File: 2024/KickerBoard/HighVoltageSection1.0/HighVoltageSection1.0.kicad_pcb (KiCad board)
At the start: 2 copper layers, 59.8 x 28.9 mm, 17 parts, among them J10 Conn_01x02_Socket, J3 Conn_01x02_Socket, J4 Conn_01x02_Socket, J6 Conn_01x02_Socket, J7 Conn_01x02_Socket, J8 Conn_01x04_Socket, J9 Conn_01x04_Socket, Q2 NMOS, Q3 NMOS

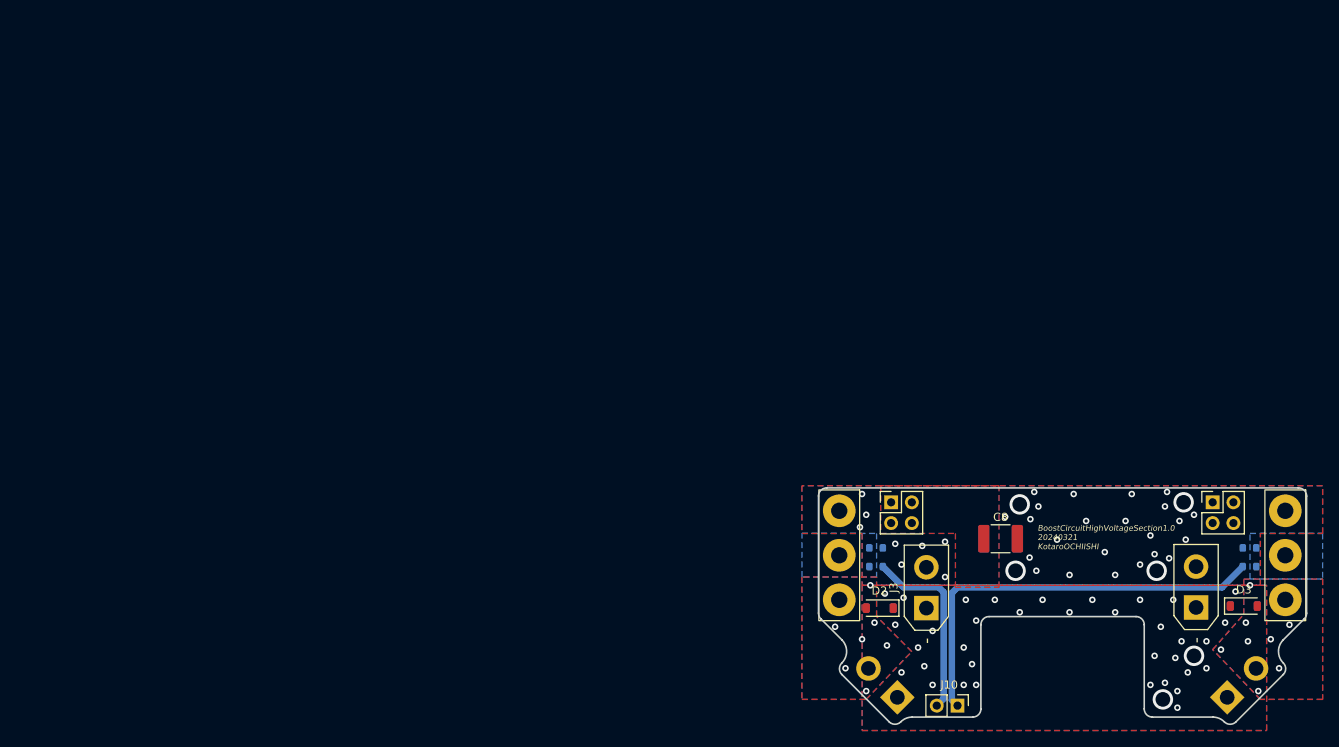
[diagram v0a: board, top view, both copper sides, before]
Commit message: add Kick&Sub
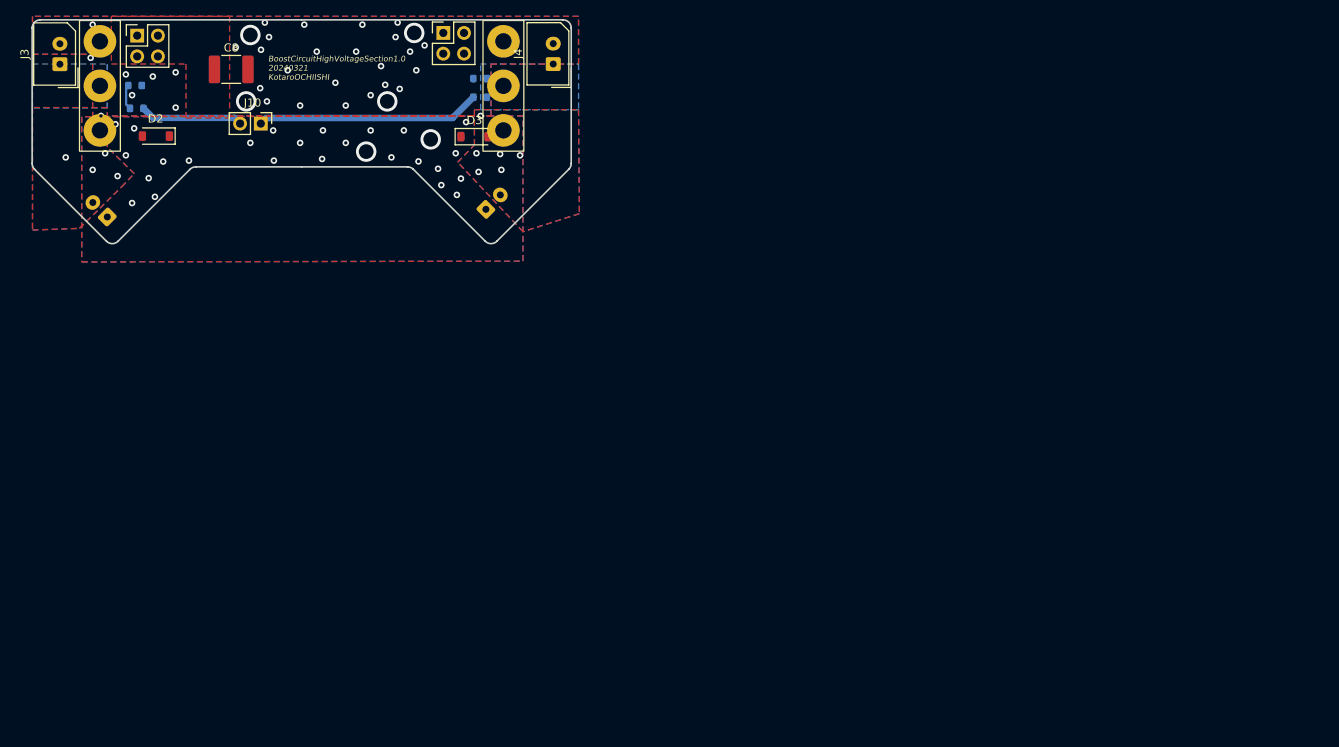
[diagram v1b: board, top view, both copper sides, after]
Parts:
- J3, J4, J6, J7: footprint Connector_AMASS:AMASS_XT30UPB-F_1x02_P5.0mm_Vertical -> Connector_Molex:Molex_SPOX_5267-02A_1x02_P2.50mm_Vertical
- moved J3 125.3 mm to (-29.6, -8.27)
- moved J6 113.2 mm to (-23.8, 10.4)
- moved Q3 111.7 mm to (24.7, -5.62)
- moved J10 111.1 mm to (-5.00, -1.00)
- moved C8 110.3 mm to (-8.63, -7.63)
- moved D3 110.3 mm to (21.1, 0.60)
- moved G*** 110.3 mm to (2.00, -5.87)
- moved J9 110.3 mm to (17.3, -12.1)
- moved R10 110.3 mm to (21.8, -4.22)
- moved R11 110.3 mm to (21.8, -6.51)
- moved J7 108.7 mm to (22.6, 9.50)
- moved J8 108.6 mm to (-20.1, -11.8)
- moved Q2 107.2 mm to (-24.7, -5.62)
- moved R9 106.9 mm to (-20.4, -5.67)
- moved R8 106.5 mm to (-20.2, -2.87)
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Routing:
- net CHIP: track 51.0 -> 27.4 mm
- net STRAIGHT: track 23.0 -> 12.6 mm
- net GATE1: track 0.00 -> 3.10 mm
- net VOUT: vias 37 -> 27
- net OUTGND2: vias 8 -> 6
- net OUTGND1: vias 7 -> 5
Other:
- board size 59.8 x 28.9 mm -> 66 x 27.4 mm

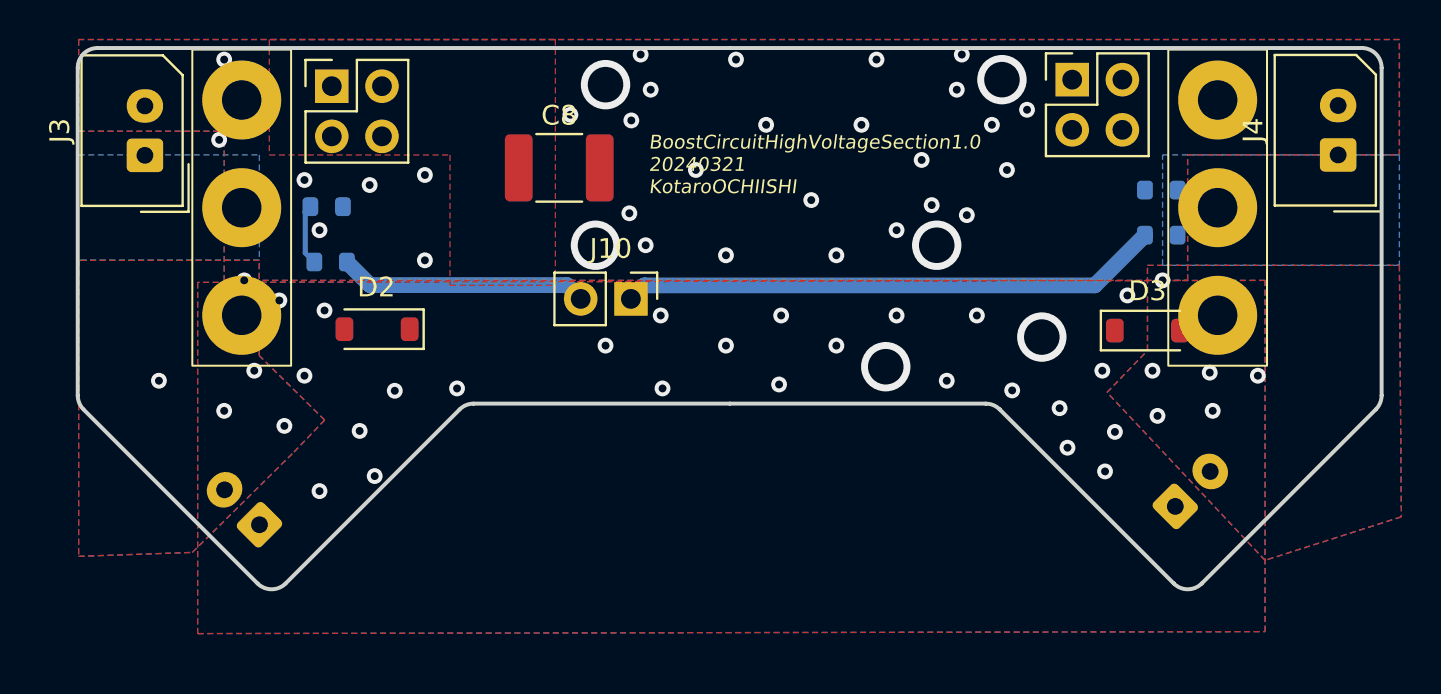
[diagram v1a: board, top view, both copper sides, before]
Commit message: add Kick&Sub
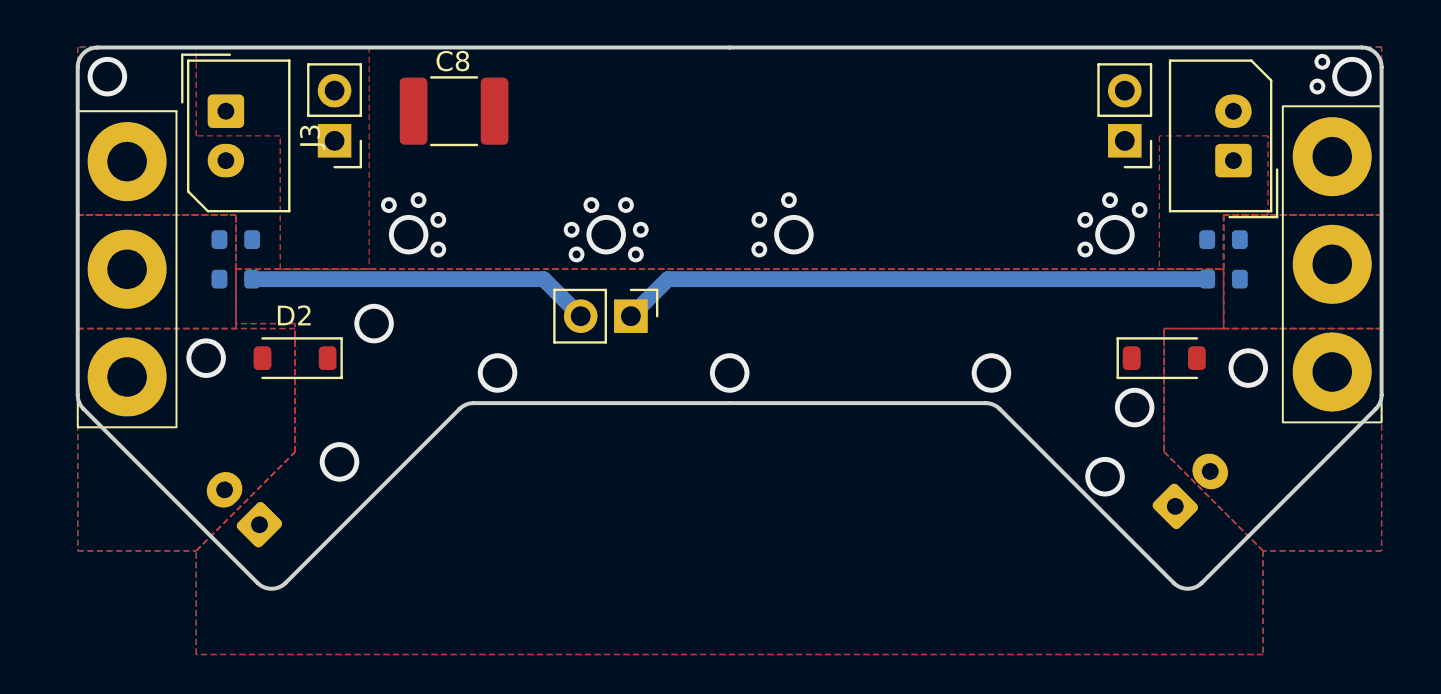
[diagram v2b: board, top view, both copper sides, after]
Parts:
- removed J10: Conn_01x02_Socket, Connector_PinHeader_2.54mm:PinHeader_1x02_P2.54mm_Vertical
- removed J8, J9: Conn_01x04_Socket, Connector_PinHeader_2.54mm:PinHeader_2x02_P2.54mm_Vertical
- added J2: Conn_01x02_Socket, Connector_PinHeader_2.54mm:PinHeader_1x02_P2.54mm_Vertical, F.Cu at (-5.00, -0.12)
- added J3: Conn_01x02_Socket, Connector_PinHeader_2.54mm:PinHeader_1x02_P2.54mm_Vertical, F.Cu at (-20.0, -9.00)
- added J4: Conn_01x02_Socket, Connector_PinHeader_2.54mm:PinHeader_1x02_P2.54mm_Vertical, F.Cu at (20.0, -9.00)
- moved G*** 9.00 mm to (11.0, -6.00)
- moved Q2 6.58 mm to (-30.5, -2.50)
- moved Q3 6.47 mm to (30.5, -2.75)
- moved C8 6.04 mm to (-13.9, -10.5)
- moved J4 5.31 mm to (25.5, -8.00)
- moved R9 4.89 mm to (-25.0, -4.00)
- moved R8 4.88 mm to (-25.0, -2.00)
- moved J3 4.67 mm to (-25.5, -10.5), turned to -90 degrees
- moved D2 4.40 mm to (-22.0, 2.00)
- moved R11 4.03 mm to (25.0, -4.00)
- moved R10 3.86 mm to (25.0, -2.00)
- moved D3 1.64 mm to (22.0, 2.00)
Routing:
- net STRAIGHT: track 12.6 -> 17.4 mm
- net GATE1: track 3.10 -> 0.00 mm
- net CHIP: track 27.4 -> 30.0 mm
- net VOUT: vias 27 -> 7
- net OUTGND2: vias 6 -> 1
- net OUTGND1: vias 5 -> 1
- net GNDPWR: vias 35 -> 25
- added copper zone on F.Cu, net GATE1
- added copper zone on F.Cu, net GATE2
